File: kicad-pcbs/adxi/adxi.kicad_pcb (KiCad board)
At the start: 4 copper layers, 106.9 x 124.1 mm, 205 parts, among them J1 FROM-PC-SPK, J10 BANDMODULE3-ANT, J11 BANDMODULE4-ANT, J12 BANDMODULE3-PA, J13 BANDMODULE4-PA, J14 BANDMODULE5-ANT, J15 BANDMODULE6-ANT, J16 BANDMODULE5-PA, J17 BANDMODULE6-PA, J18 MMCX, J2 TO-PC-MIC, J20 LCD-2004, J3 BNC, J4 SMA, J5 12V SUPPLY, J6 BANDMODULE1-ANT, J7 BANDMODULE1-PA, J8 BANDMODULE2-ANT, J9 BANDMODULE2-PA, Q1 MMBF170, Q10 HY1904C2, Q11 2N7002, Q12 HY1904C2, Q13 2N7002, Q14 HY1904C2, Q15 2N7002, Q16 HY1904C2, Q17 2N7002, Q18 HY1904C2, Q19 2N7002, Q2 HY1904C2, Q20 HY1904C2, Q21 2N7002, Q22 HY1904C2, Q23 2N7002, Q24 HY1904C2, Q25 2N7002, Q26 HY1904C2, Q3 2N7002, Q4 HY1904C2, Q5 2N7002, Q6 HY1904C2, Q63 2N7002, Q64 HY1904C2, Q7 2N7002, Q8 HY1904C2, Q9 2N7002, U1 CD2003, U3 74ACT244, U4 Si5351A-B-GT

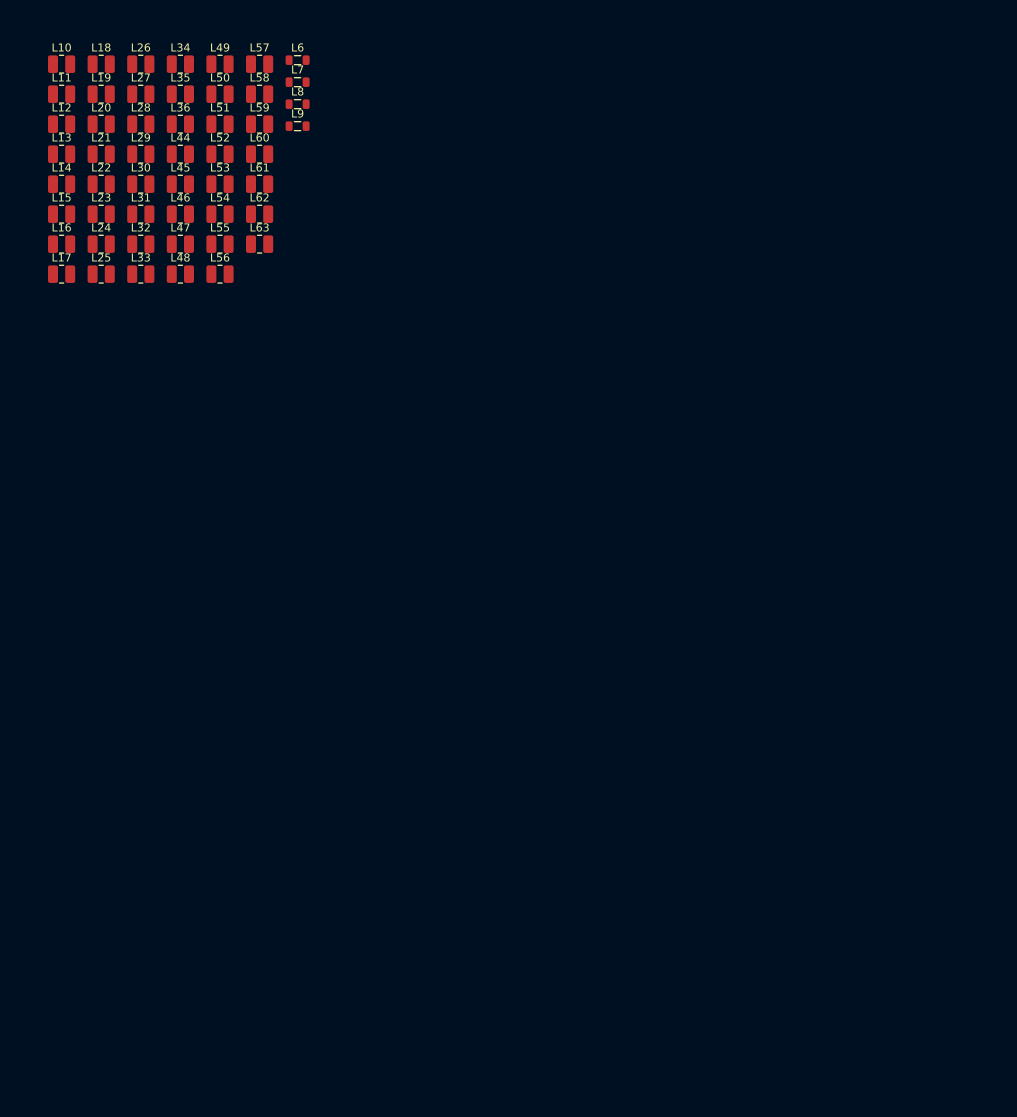
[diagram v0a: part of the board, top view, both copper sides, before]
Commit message: More outputs, etc
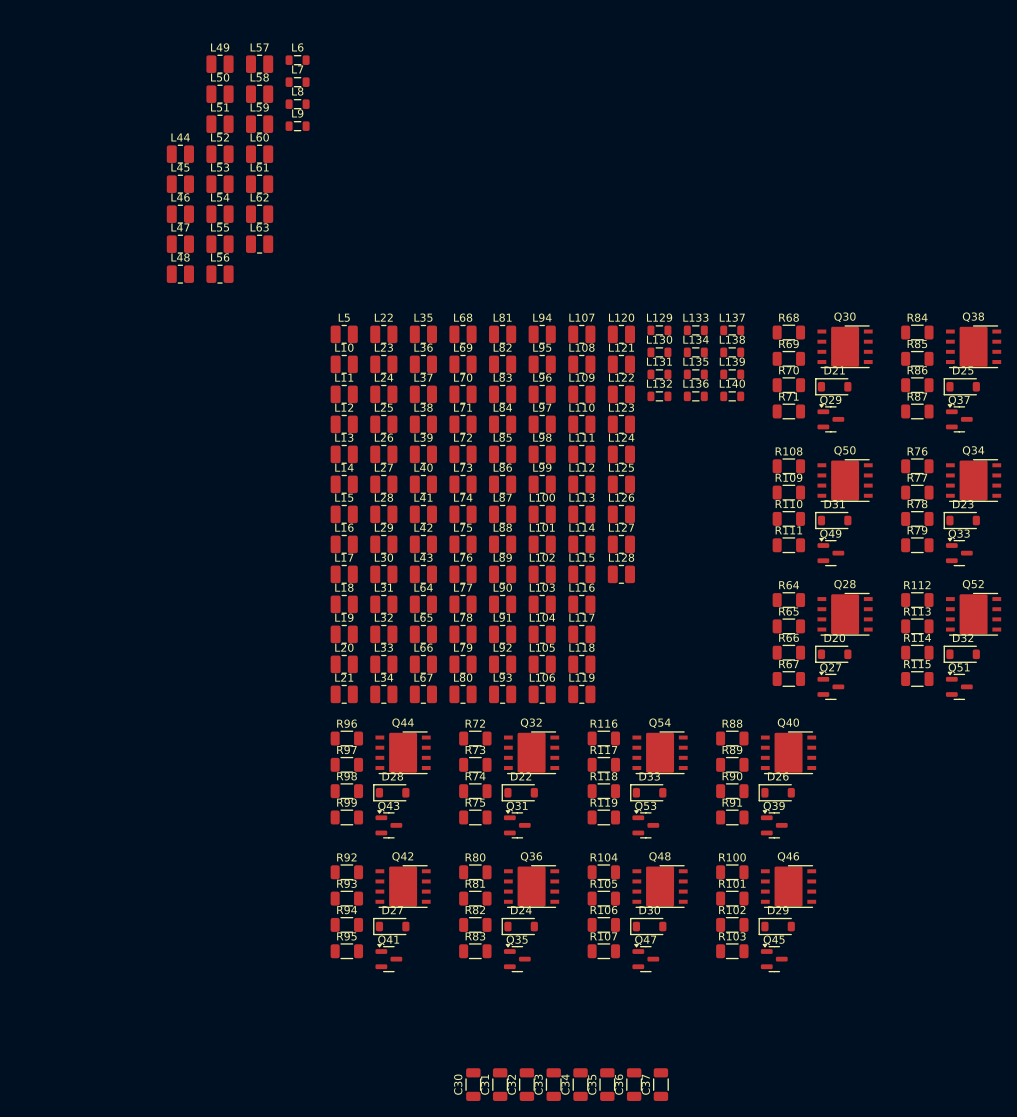
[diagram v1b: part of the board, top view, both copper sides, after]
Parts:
- added C30: 6.8pF, Capacitor_SMD:C_1206_3216Metric, F.Cu at (202.6, 157.3)
- added C31: 12pF, Capacitor_SMD:C_1206_3216Metric, F.Cu at (206.0, 157.3)
- added C32: 15pF, Capacitor_SMD:C_1206_3216Metric, F.Cu at (209.3, 157.3)
- added C33: 20pF, Capacitor_SMD:C_1206_3216Metric, F.Cu at (212.7, 157.3)
- added C34: 5.6nF, Capacitor_SMD:C_1206_3216Metric, F.Cu at (216.0, 157.3)
- added C35: 68nF, Capacitor_SMD:C_1206_3216Metric, F.Cu at (219.4, 157.3)
- added C36: 82pF, Capacitor_SMD:C_1206_3216Metric, F.Cu at (222.7, 157.3)
- added C37: 150pF, Capacitor_SMD:C_1206_3216Metric, F.Cu at (226.1, 157.3)
- added D20: BZT52C12, Diode_SMD:D_SOD-123, F.Cu at (247.8, 103.5)
- added D21: BZT52C12, Diode_SMD:D_SOD-123, F.Cu at (247.8, 70.1)
- added D22: BZT52C12, Diode_SMD:D_SOD-123, F.Cu at (208.6, 120.8)
- added D23: BZT52C12, Diode_SMD:D_SOD-123, F.Cu at (263.8, 86.8)
- added D24: BZT52C12, Diode_SMD:D_SOD-123, F.Cu at (208.6, 137.5)
- added D25: BZT52C12, Diode_SMD:D_SOD-123, F.Cu at (263.8, 70.1)
- added D26: BZT52C12, Diode_SMD:D_SOD-123, F.Cu at (240.7, 120.8)
- added D27: BZT52C12, Diode_SMD:D_SOD-123, F.Cu at (192.5, 137.5)
- added D28: BZT52C12, Diode_SMD:D_SOD-123, F.Cu at (192.5, 120.8)
- added D29: BZT52C12, Diode_SMD:D_SOD-123, F.Cu at (240.7, 137.5)
- added D30: BZT52C12, Diode_SMD:D_SOD-123, F.Cu at (224.7, 137.5)
- added D31: BZT52C12, Diode_SMD:D_SOD-123, F.Cu at (247.8, 86.8)
- added D32: BZT52C12, Diode_SMD:D_SOD-123, F.Cu at (263.8, 103.5)
- added D33: BZT52C12, Diode_SMD:D_SOD-123, F.Cu at (224.7, 120.8)
- added L100: 100nH, Inductor_SMD:L_1008_2520Metric, F.Cu at (211.2, 86.0)
- added L101: 100nH, Inductor_SMD:L_1008_2520Metric, F.Cu at (211.2, 89.8)
- added L102: 100nH, Inductor_SMD:L_1008_2520Metric, F.Cu at (211.2, 93.5)
- added L103: 100nH, Inductor_SMD:L_1008_2520Metric, F.Cu at (211.2, 97.3)
- added L104: 100nH, Inductor_SMD:L_1008_2520Metric, F.Cu at (211.2, 101.0)
- added L105: 100nH, Inductor_SMD:L_1008_2520Metric, F.Cu at (211.2, 104.8)
- added L106: 100nH, Inductor_SMD:L_1008_2520Metric, F.Cu at (211.2, 108.5)
- added L107: 100nH, Inductor_SMD:L_1008_2520Metric, F.Cu at (216.2, 63.5)
- added L108: 100nH, Inductor_SMD:L_1008_2520Metric, F.Cu at (216.2, 67.3)
- added L109: 100nH, Inductor_SMD:L_1008_2520Metric, F.Cu at (216.2, 71.0)
- added L110: 100nH, Inductor_SMD:L_1008_2520Metric, F.Cu at (216.2, 74.8)
- added L111: 100nH, Inductor_SMD:L_1008_2520Metric, F.Cu at (216.2, 78.5)
- added L112: 100nH, Inductor_SMD:L_1008_2520Metric, F.Cu at (216.2, 82.3)
- added L113: 100nH, Inductor_SMD:L_1008_2520Metric, F.Cu at (216.2, 86.0)
- added L114: 100nH, Inductor_SMD:L_1008_2520Metric, F.Cu at (216.2, 89.8)
- added L115: 100nH, Inductor_SMD:L_1008_2520Metric, F.Cu at (216.2, 93.5)
- added L116: 100nH, Inductor_SMD:L_1008_2520Metric, F.Cu at (216.2, 97.3)
- added L117: 100nH, Inductor_SMD:L_1008_2520Metric, F.Cu at (216.2, 101.0)
- added L118: 100nH, Inductor_SMD:L_1008_2520Metric, F.Cu at (216.2, 104.8)
- added L119: 100nH, Inductor_SMD:L_1008_2520Metric, F.Cu at (216.2, 108.5)
- added L120: 100nH, Inductor_SMD:L_1008_2520Metric, F.Cu at (221.1, 63.5)
- added L121: 100nH, Inductor_SMD:L_1008_2520Metric, F.Cu at (221.1, 67.3)
- added L122: 100nH, Inductor_SMD:L_1008_2520Metric, F.Cu at (221.1, 71.0)
- added L123: 100nH, Inductor_SMD:L_1008_2520Metric, F.Cu at (221.1, 74.8)
- added L124: 100nH, Inductor_SMD:L_1008_2520Metric, F.Cu at (221.1, 78.5)
- added L125: 100nH, Inductor_SMD:L_1008_2520Metric, F.Cu at (221.1, 82.3)
- added L126: 100nH, Inductor_SMD:L_1008_2520Metric, F.Cu at (221.1, 86.0)
- added L127: 100nH, Inductor_SMD:L_1008_2520Metric, F.Cu at (221.1, 89.8)
- added L128: 100nH, Inductor_SMD:L_1008_2520Metric, F.Cu at (221.1, 93.5)
- added L129: 100uH, Inductor_SMD:L_0805_2012Metric, F.Cu at (225.9, 63.0)
- added L130: 100uH, Inductor_SMD:L_0805_2012Metric, F.Cu at (225.9, 65.8)
- added L131: 100uH, Inductor_SMD:L_0805_2012Metric, F.Cu at (225.9, 68.5)
- added L132: 100uH, Inductor_SMD:L_0805_2012Metric, F.Cu at (225.9, 71.3)
- added L133: 100uH, Inductor_SMD:L_0805_2012Metric, F.Cu at (230.4, 63.0)
- added L134: 100uH, Inductor_SMD:L_0805_2012Metric, F.Cu at (230.4, 65.8)
- added L135: 100uH, Inductor_SMD:L_0805_2012Metric, F.Cu at (230.4, 68.5)
- added L136: 100uH, Inductor_SMD:L_0805_2012Metric, F.Cu at (230.4, 71.3)
- added L137: 100uH, Inductor_SMD:L_0805_2012Metric, F.Cu at (235.0, 63.0)
- added L138: 100uH, Inductor_SMD:L_0805_2012Metric, F.Cu at (235.0, 65.8)
- added L139: 100uH, Inductor_SMD:L_0805_2012Metric, F.Cu at (235.0, 68.5)
- added L140: 100uH, Inductor_SMD:L_0805_2012Metric, F.Cu at (235.0, 71.3)
- added L37: 100nH, Inductor_SMD:L_1008_2520Metric, F.Cu at (196.4, 71.0)
- added L38: 100nH, Inductor_SMD:L_1008_2520Metric, F.Cu at (196.4, 74.8)
- added L39: 100nH, Inductor_SMD:L_1008_2520Metric, F.Cu at (196.4, 78.5)
- added L40: 100nH, Inductor_SMD:L_1008_2520Metric, F.Cu at (196.4, 82.3)
- added L41: 100nH, Inductor_SMD:L_1008_2520Metric, F.Cu at (196.4, 86.0)
- added L42: 100nH, Inductor_SMD:L_1008_2520Metric, F.Cu at (196.4, 89.8)
- added L43: 100nH, Inductor_SMD:L_1008_2520Metric, F.Cu at (196.4, 93.5)
- added L5: 100nH, Inductor_SMD:L_1008_2520Metric, F.Cu at (186.5, 63.5)
- added L64: 100nH, Inductor_SMD:L_1008_2520Metric, F.Cu at (196.4, 97.3)
- added L65: 100nH, Inductor_SMD:L_1008_2520Metric, F.Cu at (196.4, 101.0)
- added L66: 100nH, Inductor_SMD:L_1008_2520Metric, F.Cu at (196.4, 104.8)
- added L67: 100nH, Inductor_SMD:L_1008_2520Metric, F.Cu at (196.4, 108.5)
- added L68: 100nH, Inductor_SMD:L_1008_2520Metric, F.Cu at (201.3, 63.5)
- added L69: 100nH, Inductor_SMD:L_1008_2520Metric, F.Cu at (201.3, 67.3)
- added L70: 100nH, Inductor_SMD:L_1008_2520Metric, F.Cu at (201.3, 71.0)
- added L71: 100nH, Inductor_SMD:L_1008_2520Metric, F.Cu at (201.3, 74.8)
- added L72: 100nH, Inductor_SMD:L_1008_2520Metric, F.Cu at (201.3, 78.5)
- added L73: 100nH, Inductor_SMD:L_1008_2520Metric, F.Cu at (201.3, 82.3)
- added L74: 100nH, Inductor_SMD:L_1008_2520Metric, F.Cu at (201.3, 86.0)
- added L75: 100nH, Inductor_SMD:L_1008_2520Metric, F.Cu at (201.3, 89.8)
- added L76: 100nH, Inductor_SMD:L_1008_2520Metric, F.Cu at (201.3, 93.5)
- added L77: 100nH, Inductor_SMD:L_1008_2520Metric, F.Cu at (201.3, 97.3)
- added L78: 100nH, Inductor_SMD:L_1008_2520Metric, F.Cu at (201.3, 101.0)
- added L79: 100nH, Inductor_SMD:L_1008_2520Metric, F.Cu at (201.3, 104.8)
- added L80: 100nH, Inductor_SMD:L_1008_2520Metric, F.Cu at (201.3, 108.5)
- added L81: 100nH, Inductor_SMD:L_1008_2520Metric, F.Cu at (206.3, 63.5)
- added L82: 100nH, Inductor_SMD:L_1008_2520Metric, F.Cu at (206.3, 67.3)
- added L83: 100nH, Inductor_SMD:L_1008_2520Metric, F.Cu at (206.3, 71.0)
- added L84: 100nH, Inductor_SMD:L_1008_2520Metric, F.Cu at (206.3, 74.8)
- added L85: 100nH, Inductor_SMD:L_1008_2520Metric, F.Cu at (206.3, 78.5)
- added L86: 100nH, Inductor_SMD:L_1008_2520Metric, F.Cu at (206.3, 82.3)
- added L87: 100nH, Inductor_SMD:L_1008_2520Metric, F.Cu at (206.3, 86.0)
- added L88: 100nH, Inductor_SMD:L_1008_2520Metric, F.Cu at (206.3, 89.8)
- added L89: 100nH, Inductor_SMD:L_1008_2520Metric, F.Cu at (206.3, 93.5)
- added L90: 100nH, Inductor_SMD:L_1008_2520Metric, F.Cu at (206.3, 97.3)
- added L91: 100nH, Inductor_SMD:L_1008_2520Metric, F.Cu at (206.3, 101.0)
- added L92: 100nH, Inductor_SMD:L_1008_2520Metric, F.Cu at (206.3, 104.8)
- added L93: 100nH, Inductor_SMD:L_1008_2520Metric, F.Cu at (206.3, 108.5)
- added L94: 100nH, Inductor_SMD:L_1008_2520Metric, F.Cu at (211.2, 63.5)
- added L95: 100nH, Inductor_SMD:L_1008_2520Metric, F.Cu at (211.2, 67.3)
- added L96: 100nH, Inductor_SMD:L_1008_2520Metric, F.Cu at (211.2, 71.0)
- added L97: 100nH, Inductor_SMD:L_1008_2520Metric, F.Cu at (211.2, 74.8)
- added L98: 100nH, Inductor_SMD:L_1008_2520Metric, F.Cu at (211.2, 78.5)
- added L99: 100nH, Inductor_SMD:L_1008_2520Metric, F.Cu at (211.2, 82.3)
- added Q27: 2N7002, Package_TO_SOT_SMD:SOT-23, F.Cu at (247.3, 107.6)
- added Q28: HY1904C2, kicad-parts:HY1904C2, F.Cu at (249.1, 98.5)
- added Q29: 2N7002, Package_TO_SOT_SMD:SOT-23, F.Cu at (247.3, 74.2)
- added Q30: HY1904C2, kicad-parts:HY1904C2, F.Cu at (249.1, 65.1)
- added Q31: 2N7002, Package_TO_SOT_SMD:SOT-23, F.Cu at (208.1, 124.9)
- added Q32: HY1904C2, kicad-parts:HY1904C2, F.Cu at (209.9, 115.8)
- added Q33: 2N7002, Package_TO_SOT_SMD:SOT-23, F.Cu at (263.4, 90.9)
- added Q34: HY1904C2, kicad-parts:HY1904C2, F.Cu at (265.2, 81.8)
- added Q35: 2N7002, Package_TO_SOT_SMD:SOT-23, F.Cu at (208.1, 141.6)
- added Q36: HY1904C2, kicad-parts:HY1904C2, F.Cu at (209.9, 132.5)
- added Q37: 2N7002, Package_TO_SOT_SMD:SOT-23, F.Cu at (263.4, 74.2)
- added Q38: HY1904C2, kicad-parts:HY1904C2, F.Cu at (265.2, 65.1)
- added Q39: 2N7002, Package_TO_SOT_SMD:SOT-23, F.Cu at (240.2, 124.9)
- added Q40: HY1904C2, kicad-parts:HY1904C2, F.Cu at (242.0, 115.8)
- added Q41: 2N7002, Package_TO_SOT_SMD:SOT-23, F.Cu at (192.1, 141.6)
- added Q42: HY1904C2, kicad-parts:HY1904C2, F.Cu at (193.8, 132.5)
- added Q43: 2N7002, Package_TO_SOT_SMD:SOT-23, F.Cu at (192.1, 124.9)
- added Q44: HY1904C2, kicad-parts:HY1904C2, F.Cu at (193.8, 115.8)
- added Q45: 2N7002, Package_TO_SOT_SMD:SOT-23, F.Cu at (240.2, 141.6)
- added Q46: HY1904C2, kicad-parts:HY1904C2, F.Cu at (242.0, 132.5)
- added Q47: 2N7002, Package_TO_SOT_SMD:SOT-23, F.Cu at (224.2, 141.6)
- added Q48: HY1904C2, kicad-parts:HY1904C2, F.Cu at (226.0, 132.5)
- added Q49: 2N7002, Package_TO_SOT_SMD:SOT-23, F.Cu at (247.3, 90.9)
- added Q50: HY1904C2, kicad-parts:HY1904C2, F.Cu at (249.1, 81.8)
- added Q51: 2N7002, Package_TO_SOT_SMD:SOT-23, F.Cu at (263.4, 107.6)
- added Q52: HY1904C2, kicad-parts:HY1904C2, F.Cu at (265.2, 98.5)
- added Q53: 2N7002, Package_TO_SOT_SMD:SOT-23, F.Cu at (224.2, 124.9)
- added Q54: HY1904C2, kicad-parts:HY1904C2, F.Cu at (226.0, 115.8)
- added R100: 1K 0.25W, Resistor_SMD:R_1206_3216Metric, F.Cu at (235.0, 130.8)
- added R101: 6.8K 0.25W, Resistor_SMD:R_1206_3216Metric, F.Cu at (235.0, 134.1)
- added R102: 6.8K 0.25W, Resistor_SMD:R_1206_3216Metric, F.Cu at (235.0, 137.3)
- added R103: 1K 0.25W, Resistor_SMD:R_1206_3216Metric, F.Cu at (235.0, 140.6)
- added R104: 1K 0.25W, Resistor_SMD:R_1206_3216Metric, F.Cu at (218.9, 130.8)
- added R105: 6.8K 0.25W, Resistor_SMD:R_1206_3216Metric, F.Cu at (218.9, 134.1)
- added R106: 6.8K 0.25W, Resistor_SMD:R_1206_3216Metric, F.Cu at (218.9, 137.3)
- added R107: 1K 0.25W, Resistor_SMD:R_1206_3216Metric, F.Cu at (218.9, 140.6)
- added R108: 1K 0.25W, Resistor_SMD:R_1206_3216Metric, F.Cu at (242.1, 80.0)
- added R109: 6.8K 0.25W, Resistor_SMD:R_1206_3216Metric, F.Cu at (242.1, 83.3)
- added R110: 6.8K 0.25W, Resistor_SMD:R_1206_3216Metric, F.Cu at (242.1, 86.6)
- added R111: 1K 0.25W, Resistor_SMD:R_1206_3216Metric, F.Cu at (242.1, 89.9)
- added R112: 1K 0.25W, Resistor_SMD:R_1206_3216Metric, F.Cu at (258.1, 96.7)
- added R113: 6.8K 0.25W, Resistor_SMD:R_1206_3216Metric, F.Cu at (258.1, 100.0)
- added R114: 6.8K 0.25W, Resistor_SMD:R_1206_3216Metric, F.Cu at (258.1, 103.3)
- added R115: 1K 0.25W, Resistor_SMD:R_1206_3216Metric, F.Cu at (258.1, 106.6)
- added R116: 1K 0.25W, Resistor_SMD:R_1206_3216Metric, F.Cu at (218.9, 114.0)
- added R117: 6.8K 0.25W, Resistor_SMD:R_1206_3216Metric, F.Cu at (218.9, 117.3)
- added R118: 6.8K 0.25W, Resistor_SMD:R_1206_3216Metric, F.Cu at (218.9, 120.6)
- added R119: 1K 0.25W, Resistor_SMD:R_1206_3216Metric, F.Cu at (218.9, 123.9)
- added R64: 1K 0.25W, Resistor_SMD:R_1206_3216Metric, F.Cu at (242.1, 96.7)
- added R65: 6.8K 0.25W, Resistor_SMD:R_1206_3216Metric, F.Cu at (242.1, 100.0)
- added R66: 6.8K 0.25W, Resistor_SMD:R_1206_3216Metric, F.Cu at (242.1, 103.3)
- added R67: 1K 0.25W, Resistor_SMD:R_1206_3216Metric, F.Cu at (242.1, 106.6)
- added R68: 1K 0.25W, Resistor_SMD:R_1206_3216Metric, F.Cu at (242.1, 63.3)
- added R69: 6.8K 0.25W, Resistor_SMD:R_1206_3216Metric, F.Cu at (242.1, 66.6)
- added R70: 6.8K 0.25W, Resistor_SMD:R_1206_3216Metric, F.Cu at (242.1, 69.9)
- added R71: 1K 0.25W, Resistor_SMD:R_1206_3216Metric, F.Cu at (242.1, 73.2)
- added R72: 1K 0.25W, Resistor_SMD:R_1206_3216Metric, F.Cu at (202.9, 114.0)
- added R73: 6.8K 0.25W, Resistor_SMD:R_1206_3216Metric, F.Cu at (202.9, 117.3)
- added R74: 6.8K 0.25W, Resistor_SMD:R_1206_3216Metric, F.Cu at (202.9, 120.6)
- added R75: 1K 0.25W, Resistor_SMD:R_1206_3216Metric, F.Cu at (202.9, 123.9)
- added R76: 1K 0.25W, Resistor_SMD:R_1206_3216Metric, F.Cu at (258.1, 80.0)
- added R77: 6.8K 0.25W, Resistor_SMD:R_1206_3216Metric, F.Cu at (258.1, 83.3)
- added R78: 6.8K 0.25W, Resistor_SMD:R_1206_3216Metric, F.Cu at (258.1, 86.6)
- added R79: 1K 0.25W, Resistor_SMD:R_1206_3216Metric, F.Cu at (258.1, 89.9)
- added R80: 1K 0.25W, Resistor_SMD:R_1206_3216Metric, F.Cu at (202.9, 130.8)
- added R81: 6.8K 0.25W, Resistor_SMD:R_1206_3216Metric, F.Cu at (202.9, 134.1)
- added R82: 6.8K 0.25W, Resistor_SMD:R_1206_3216Metric, F.Cu at (202.9, 137.3)
- added R83: 1K 0.25W, Resistor_SMD:R_1206_3216Metric, F.Cu at (202.9, 140.6)
- added R84: 1K 0.25W, Resistor_SMD:R_1206_3216Metric, F.Cu at (258.1, 63.3)
- added R85: 6.8K 0.25W, Resistor_SMD:R_1206_3216Metric, F.Cu at (258.1, 66.6)
- added R86: 6.8K 0.25W, Resistor_SMD:R_1206_3216Metric, F.Cu at (258.1, 69.9)
- added R87: 1K 0.25W, Resistor_SMD:R_1206_3216Metric, F.Cu at (258.1, 73.2)
- added R88: 1K 0.25W, Resistor_SMD:R_1206_3216Metric, F.Cu at (235.0, 114.0)
- added R89: 6.8K 0.25W, Resistor_SMD:R_1206_3216Metric, F.Cu at (235.0, 117.3)
- added R90: 6.8K 0.25W, Resistor_SMD:R_1206_3216Metric, F.Cu at (235.0, 120.6)
- added R91: 1K 0.25W, Resistor_SMD:R_1206_3216Metric, F.Cu at (235.0, 123.9)
- added R92: 1K 0.25W, Resistor_SMD:R_1206_3216Metric, F.Cu at (186.8, 130.8)
- added R93: 6.8K 0.25W, Resistor_SMD:R_1206_3216Metric, F.Cu at (186.8, 134.1)
- added R94: 6.8K 0.25W, Resistor_SMD:R_1206_3216Metric, F.Cu at (186.8, 137.3)
- added R95: 1K 0.25W, Resistor_SMD:R_1206_3216Metric, F.Cu at (186.8, 140.6)
- added R96: 1K 0.25W, Resistor_SMD:R_1206_3216Metric, F.Cu at (186.8, 114.0)
- added R97: 6.8K 0.25W, Resistor_SMD:R_1206_3216Metric, F.Cu at (186.8, 117.3)
- added R98: 6.8K 0.25W, Resistor_SMD:R_1206_3216Metric, F.Cu at (186.8, 120.6)
- added R99: 1K 0.25W, Resistor_SMD:R_1206_3216Metric, F.Cu at (186.8, 123.9)
- L10, L11, L12, L13, L14, L15, L16, L17, L18, L19, L20, L21, L22, L23, L24, L25, L26, L27, L28, L29, L30, L31, L32, L33, L34, L35, L36: value 3.3uH -> 100nH
- moved L34 82.8 mm to (191.4, 108.5)
- moved L18 74.0 mm to (186.5, 97.3)
- moved L19 74.0 mm to (186.5, 101.0)
- moved L20 74.0 mm to (186.5, 104.8)
- moved L21 74.0 mm to (186.5, 108.5)
- moved L26 57.5 mm to (191.4, 78.5)
- moved L27 57.5 mm to (191.4, 82.3)
- moved L28 57.5 mm to (191.4, 86.0)
- moved L29 57.5 mm to (191.4, 89.8)
- moved L30 57.5 mm to (191.4, 93.5)
- moved L31 57.5 mm to (191.4, 97.3)
- moved L32 57.5 mm to (191.4, 101.0)
- moved L33 57.5 mm to (191.4, 104.8)
- moved L10 51.5 mm to (186.5, 67.3)
- moved L11 51.5 mm to (186.5, 71.0)
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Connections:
- net /PA Switched RF Choke/L-100UH-A renamed /PA Switched Resonator/L-100UH-A
- net /PA Switched RF Choke/L-100UH-B renamed Net-(L131-Pad2)
- net /PA Switched RF Choke/L-50UH-A renamed /PA Switched Resonator/L-50UH-A
- net /PA Switched RF Choke/L-50UH-B renamed /PA Switched Resonator/L-50UH-B
- L10 pad 1: Net-(L10-Pad1) -> /PA Switched Resonator/L-10UH-A
- L11 pad 1: Net-(L10-Pad2) -> /PA Switched Resonator/L-10UH-A
- L11 pad 2: Net-(L11-Pad2) -> Net-(L10-Pad2)
- L12 pad 1: Net-(L11-Pad2) -> /PA Switched Resonator/L-10UH-A
- L12 pad 2: Net-(L12-Pad2) -> Net-(L10-Pad2)
- L13 pad 1: Net-(L12-Pad2) -> Net-(L10-Pad2)
- L14 pad 1: /PA Switched RF Choke/L-10UH-A -> Net-(L10-Pad2)
- L14 pad 2: Net-(L14-Pad2) -> Net-(L13-Pad2)
- L15 pad 1: /PA Switched RF Choke/L-10UH-A -> Net-(L10-Pad2)
- L15 pad 2: Net-(L14-Pad2) -> Net-(L13-Pad2)
- L16 pad 1: /PA Switched RF Choke/L-10UH-A -> Net-(L10-Pad2)
- L16 pad 2: Net-(L14-Pad2) -> Net-(L13-Pad2)
- L17 pad 1: Net-(L14-Pad2) -> Net-(L10-Pad2)
- L17 pad 2: Net-(L17-Pad2) -> Net-(L13-Pad2)
- L18 pad 1: Net-(L14-Pad2) -> Net-(L13-Pad2)
- L18 pad 2: Net-(L17-Pad2) -> Net-(L18-Pad2)
- L19 pad 1: Net-(L14-Pad2) -> Net-(L13-Pad2)
- L19 pad 2: Net-(L17-Pad2) -> Net-(L18-Pad2)
- L20 pad 1: Net-(L17-Pad2) -> Net-(L13-Pad2)
- L20 pad 2: Net-(L10-Pad1) -> Net-(L18-Pad2)
- L21 pad 1: Net-(L17-Pad2) -> Net-(L13-Pad2)
- L21 pad 2: Net-(L10-Pad1) -> Net-(L18-Pad2)
- L22 pad 1: Net-(L17-Pad2) -> Net-(L13-Pad2)
- L22 pad 2: Net-(L10-Pad1) -> Net-(L18-Pad2)
- L23 pad 1: Net-(L13-Pad2) -> Net-(L18-Pad2)
- L24 pad 1: Net-(L23-Pad2) -> Net-(L18-Pad2)
- L24 pad 2: /PA Switched RF Choke/L-10UH-B -> Net-(L23-Pad2)
- L25 pad 1: Net-(L10-Pad1) -> Net-(L18-Pad2)
- L25 pad 2: Net-(L10-Pad2) -> Net-(L23-Pad2)
- L26 pad 1: Net-(L10-Pad2) -> Net-(L18-Pad2)
- L26 pad 2: Net-(L11-Pad2) -> Net-(L23-Pad2)
- L27 pad 1: Net-(L11-Pad2) -> Net-(L18-Pad2)
- L27 pad 2: Net-(L12-Pad2) -> Net-(L23-Pad2)
- L28 pad 1: Net-(L12-Pad2) -> Net-(L23-Pad2)
- L28 pad 2: Net-(L13-Pad2) -> Net-(L28-Pad2)
- L29 pad 1: Net-(L13-Pad2) -> Net-(L23-Pad2)
- L29 pad 2: Net-(L23-Pad2) -> Net-(L28-Pad2)
- L30 pad 2: /PA Switched RF Choke/L-10UH-B -> Net-(L28-Pad2)
- L31 pad 1: Net-(L10-Pad1) -> Net-(L23-Pad2)
- L31 pad 2: Net-(L10-Pad2) -> Net-(L28-Pad2)
- L32 pad 1: Net-(L10-Pad2) -> Net-(L23-Pad2)
- L32 pad 2: Net-(L11-Pad2) -> Net-(L28-Pad2)
- L33 pad 1: Net-(L11-Pad2) -> Net-(L28-Pad2)
- L33 pad 2: Net-(L12-Pad2) -> Net-(L33-Pad2)
- L34 pad 1: Net-(L12-Pad2) -> Net-(L28-Pad2)
- L34 pad 2: Net-(L13-Pad2) -> Net-(L33-Pad2)
- L35 pad 1: Net-(L13-Pad2) -> Net-(L28-Pad2)
- L35 pad 2: Net-(L23-Pad2) -> Net-(L33-Pad2)
- L36 pad 1: Net-(L23-Pad2) -> Net-(L28-Pad2)
- L36 pad 2: /PA Switched RF Choke/L-10UH-B -> Net-(L33-Pad2)
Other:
- board text added: "5 TIER CHINESE TIFFIN LUNCH BOX"
- board text added: "ATU/ANT OUT LPF/SWR DISPLAY PA/RF CHOKE MCU/TIMING PSU"
- board text added: "POTENTIAL TIERS:"
- board text added: "https://duckduckgo.com/?q=hellema+spiced+cookies+tin"
- board text added: "https://www.aliexpress.com/item/1005006756495960.html https://www.aliexpress.com/item/1005006075889043.html"
- board text added: "https://www.aliexpress.com/item/1005006978580242.html"
